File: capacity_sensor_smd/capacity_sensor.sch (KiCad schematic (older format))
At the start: 37 parts, among them J1 TP1, J2 Sensor, J3 TP2, J4 TP3, J5 Polarity, J6 TP4, J7 Pwr/Out, P1 Prot. Diode, Q1 2N2222, U1 ICM7555, U2 74HCT14, U3 74HC74

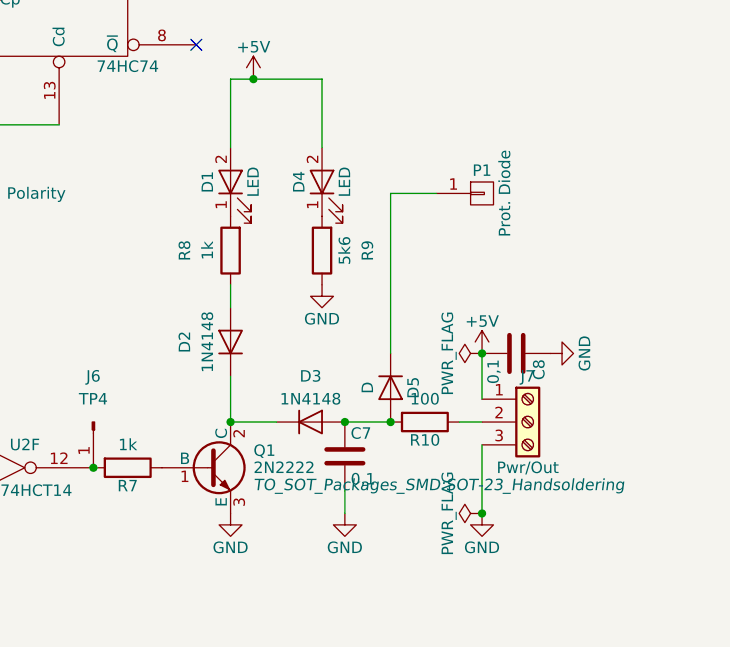
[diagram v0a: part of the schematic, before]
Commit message: template
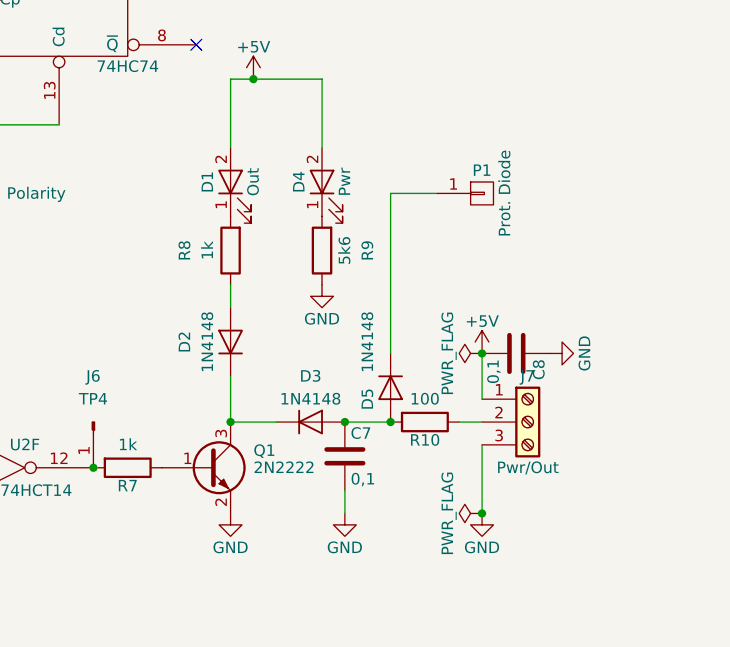
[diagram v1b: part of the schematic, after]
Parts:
- removed Q1: 2N2222, TO_SOT_Packages_SMD:SOT-23_Handsoldering, symbol PZT2222A
- added Q1: 2N2222, TO_SOT_Packages_SMD:SOT-23_Handsoldering, symbol 2N3055
- D1: value LED -> Out
- D4: value LED -> Pwr
- D5: value D -> 1N4148
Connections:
- net GND: now also Q1.2 (E)
- net at R7.1: now also Q1.1 (B)
- net at D2.1 (K), D3.1 (K): now also Q1.3 (C)
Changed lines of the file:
@@
 P 9500 1950
 F 0 "D1" H 9500 2050 50  0000 C CNN
-F 1 "LED" H 9500 1850 50  0000 C CNN
+F 1 "Out" H 9500 1850 50  0000 C CNN
 F 2 "LEDs:LED_1206_HandSoldering" H 9500 1950 50  0001 C CNN
 F 3 "" H 9500 1950 50  0000 C CNN
@@
 P 9900 1950
 F 0 "D4" H 9900 2050 50  0000 C CNN
-F 1 "LED" H 9900 1850 50  0000 C CNN
+F 1 "Pwr" H 9900 1850 50  0000 C CNN
 F 2 "LEDs:LED_1206_HandSoldering" H 9900 1950 50  0001 C CNN
 F 3 "" H 9900 1950 50  0000 C CNN
@@
 Connection ~ 9600 1500
 $Comp
-L PZT2222A Q1
-U 1 1 5A5F8CA7
-P 9400 3200
-F 0 "Q1" H 9600 3275 50  0000 L CNN
-F 1 "2N2222" H 9600 3200 50  0000 L CNN
-F 2 "TO_SOT_Packages_SMD:SOT-23_Handsoldering" H 9600 3125 50  0000 L CIN
-F 3 "" H 9400 3200 50  0000 L CNN
-	1    9400 3200
-	1    0    0    -1
-$EndComp
-$Comp
 L D D5
 U 1 1 5A5F8E01
 P 10200 2850
-F 0 "D5" H 10200 2950 50  0000 C CNN
-F 1 "D" H 10200 2750 50  0000 C CNN
+F 0 "D5" H 10250 2750 50  0000 C CNN
+F 1 "1N4148" H 10000 2750 50  0000 C CNN
 F 2 "Diodes_SMD:D_PowerDI-123" H 10200 2850 50  0001 C CNN
 F 3 "" H 10200 2850 50  0000 C CNN
@@
 Wire Wire Line
 	6800 1600 6900 1600
+$Comp
+L 2N3055 Q1
+U 1 1 5AD1BD32
+P 9400 3200
+F 0 "Q1" H 9600 3275 50  0000 L CNN
+F 1 "2N2222" H 9600 3200 50  0000 L CNN
+F 2 "TO_SOT_Packages_SMD:SOT-23_Handsoldering" H 9600 3125 50  0001 L CIN
+F 3 "" H 9400 3200 50  0001 L CNN
+	1    9400 3200
+	1    0    0    -1
+$EndComp
 $EndSCHEMATC
